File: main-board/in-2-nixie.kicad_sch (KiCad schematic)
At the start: 26 parts, among them J1 Encoder, J2 Matrix, J3 Power, J4 DS3231, J5 Buttons, T1 IN-2, T2 IN-2, T3 IN-2, T4 IN-2, U1 HV5222PJ, U2 Nixie HVPS, U3 ESP32-C6 SuperMini, U4 Level Shifter

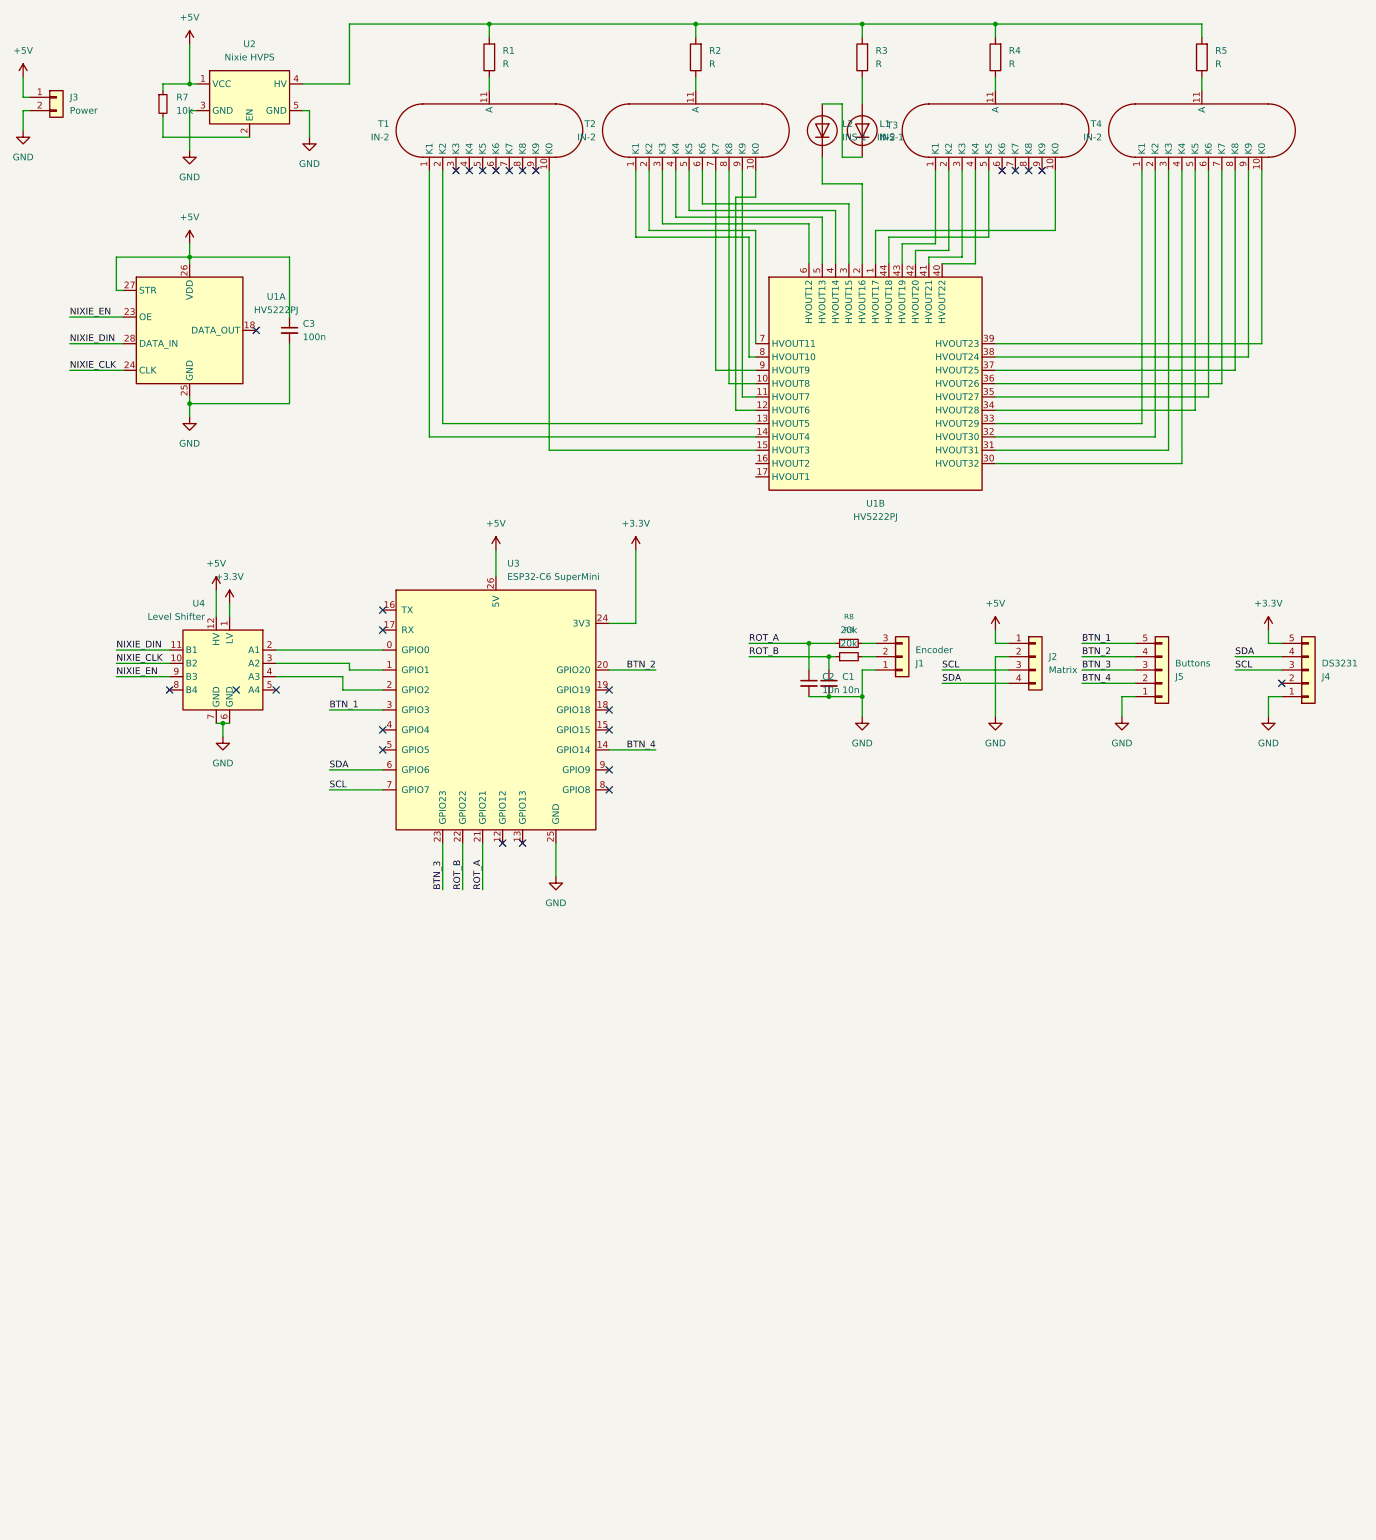
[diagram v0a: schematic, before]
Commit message: pcb
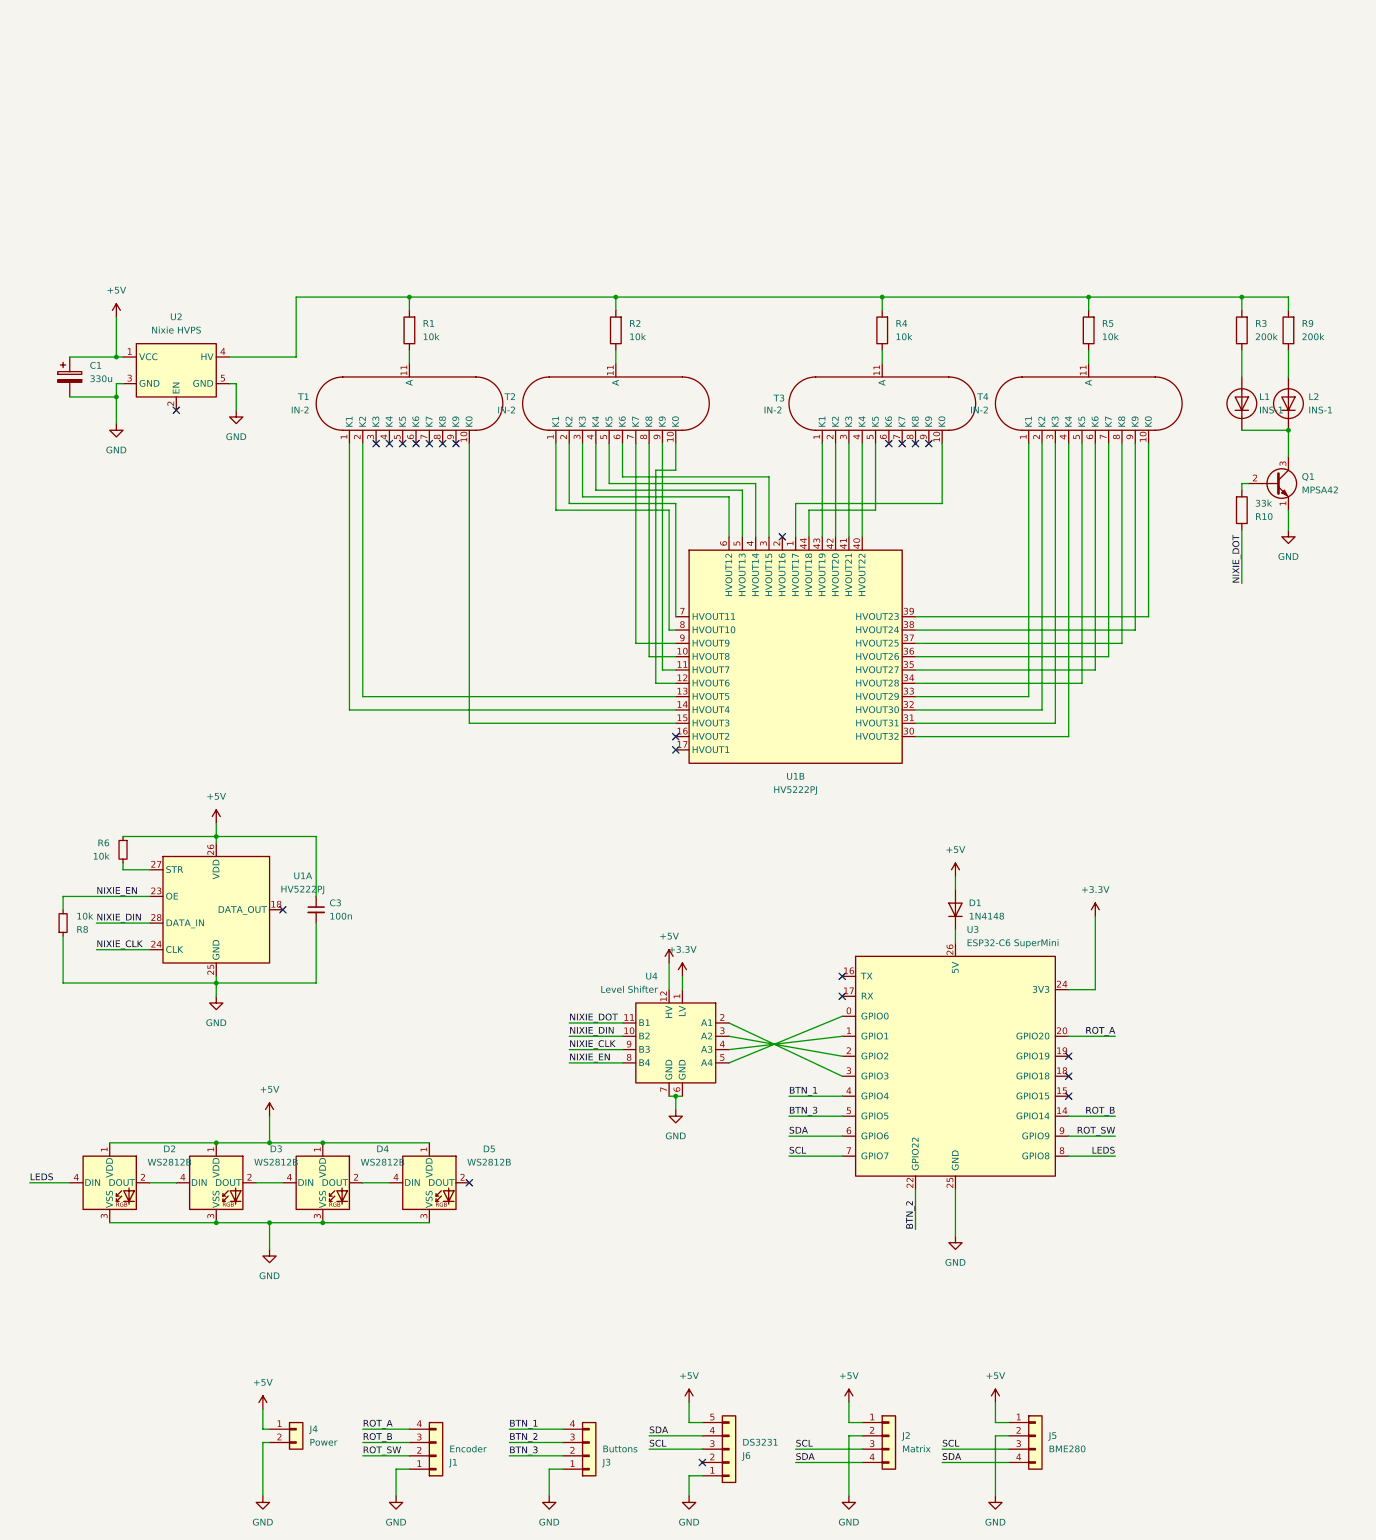
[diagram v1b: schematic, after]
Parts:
- removed C1, C2: 10n, Capacitor_THT:C_Disc_D5.0mm_W2.5mm_P5.00mm, symbol Device:C_Small
- removed J4: DS3231, Connector_PinHeader_2.54mm:PinHeader_1x05_P2.54mm_Vertical, symbol Connector_Generic:Conn_01x05
- removed R7: 10k, Resistor_THT:R_Axial_DIN0207_L6.3mm_D2.5mm_P7.62mm_Horizontal, symbol Device:R_Small
- removed R9: 20k, Resistor_THT:R_Axial_DIN0207_L6.3mm_D2.5mm_P7.62mm_Horizontal, symbol Device:R_Small
- added C1: 330u, Capacitor_THT:CP_Radial_D8.0mm_P3.50mm, symbol Device:C_Polarized
- added D1: 1N4148, Diode_THT:D_DO-35_SOD27_P7.62mm_Horizontal, symbol Diode:1N4148
- added D2, D3, D4, D5: WS2812B, in-2-nixie:APA106_D5-Staggered_Pins, symbol LED:WS2812B
- added J5: BME280, Connector_PinHeader_2.54mm:PinHeader_1x04_P2.54mm_Vertical, symbol Connector_Generic:Conn_01x04
- added J6: DS3231, Connector_PinHeader_2.54mm:PinHeader_1x05_P2.54mm_Vertical, symbol Connector_Generic:Conn_01x05
- added Q1: MPSA42, Package_TO_SOT_THT:TO-92_Inline, symbol Transistor_BJT:MPSA42
- added R10: 33k, Resistor_THT:R_Axial_DIN0207_L6.3mm_D2.5mm_P2.54mm_Vertical, symbol Device:R
- added R6: 10k, Resistor_THT:R_Axial_DIN0207_L6.3mm_D2.5mm_P2.54mm_Vertical, symbol Device:R_Small
- added R9: 200k, Resistor_THT:R_Axial_DIN0207_L6.3mm_D2.5mm_P7.62mm_Horizontal, symbol Device:R
- J1: footprint Connector_PinHeader_2.54mm:PinHeader_1x03_P2.54mm_Vertical -> Connector_PinHeader_2.54mm:PinHeader_1x04_P2.54mm_Vertical; symbol Connector_Generic:Conn_01x03 -> Connector_Generic:Conn_01x04
- J3: renamed from J5; footprint Connector_PinHeader_2.54mm:PinHeader_1x05_P2.54mm_Vertical -> Connector_PinHeader_2.54mm:PinHeader_1x04_P2.54mm_Vertical; symbol Connector_Generic:Conn_01x05 -> Connector_Generic:Conn_01x04
- R1, R2, R4, R5: value R -> 10k
- R3: value R -> 200k
- R8: value 20k -> 10k; footprint Resistor_THT:R_Axial_DIN0207_L6.3mm_D2.5mm_P7.62mm_Horizontal -> Resistor_THT:R_Axial_DIN0207_L6.3mm_D2.5mm_P2.54mm_Vertical
- T1, T2, T3: footprint in-2-nixie:IN-2 Nixie Tube -> in-2-nixie:IN-2 Nixie Tube (w. pins)
- U1: footprint Package_LCC:PLCC-44_16.6x16.6mm_P1.27mm -> in-2-nixie:PLCC-44 LongPads
- renumbered J3 to J4
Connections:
- net +5V: now also C1.1, D1.2 (A), D2.1 (VDD), D3.1 (VDD), D4.1 (VDD), D5.1 (VDD), J5.1 (Pin_1), J6.5 (Pin_5), R6.1; no longer U1.27 (STR), U3.26 (5V)
- net BTN_1: now also J3.4 (Pin_4), U3.4 (GPIO4); no longer J3.5 (Pin_5), U3.3 (GPIO3)
- net BTN_2: now also J3.3 (Pin_3), U3.22 (GPIO22); no longer J3.4 (Pin_4), U3.20 (GPIO20)
- net BTN_3: now also J3.2 (Pin_2), U3.5 (GPIO5); no longer J3.3 (Pin_3), U3.23 (GPIO23)
- net GND: now also R8.1, C1.2, D2.3 (VSS), D3.3 (VSS), D4.3 (VSS), D5.3 (VSS), J5.2 (Pin_2), J6.1 (Pin_1), Q1.1 (E)
- net NIXIE_CLK: now also U4.9 (B3); no longer U4.10 (B2)
- net NIXIE_DIN: now also U4.10 (B2); no longer U4.11 (B1)
- net NIXIE_EN: now also R8.2, U4.8 (B4); no longer U4.9 (B3)
- net ROT_A: now also J1.4 (Pin_4), U3.20 (GPIO20); no longer R8.1, U3.21 (GPIO21)
- net ROT_B: now also J1.3 (Pin_3), U3.14 (GPIO14); no longer U3.22 (GPIO22)
- net SCL: now also J5.3 (Pin_3), J6.3 (Pin_3)
- net SDA: now also J5.4 (Pin_4), J6.4 (Pin_4)
- net ROT_SW: now reaches J1.2 (Pin_2)
- net ROT_SW: now also U3.9 (GPIO9)
- net at R1.2, R2.2, R3.2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: now also R9.2
- net at L2.1 (K): now also L1.1 (K), Q1.3 (C); no longer U1.2 (HVOUT16)
- net at L2.2 (A): now also R9.1; no longer L1.1 (K)
- net at U4.2 (A1): now also U3.3 (GPIO3); no longer U3.0 (GPIO0)
- net at U4.3 (A2): now also U3.2 (GPIO2); no longer U3.1 (GPIO1)
- net at U4.4 (A3): now also U3.1 (GPIO1); no longer U3.2 (GPIO2)
- net at U4.5 (A4): now also U3.0 (GPIO0)
- net LEDS: now reaches U3.8 (GPIO8)
- net LEDS: now also D2.4 (DIN)
- removed net BTN_4: J3.2 (Pin_2), U3.14 (GPIO14)
- new net: D3.2 (DOUT), D4.4 (DIN)
- new net: D2.2 (DOUT), D3.4 (DIN)
- new net: D4.2 (DOUT), D5.4 (DIN)
- new net: Q1.2 (B), R10.2
- new net: D1.1 (K), U3.26 (5V)
- new net: R6.2, U1.27 (STR)
- new net NIXIE_DOT: R10.1, U4.11 (B1)
- no-connect marks 27 -> 23
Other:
- moved on the sheet: C3, J2, J4, L1, L2, R1, R2, R3, R4, R5, T1, T2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
